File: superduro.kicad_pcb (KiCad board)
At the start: 2 copper layers, 21.6 x 24.1 mm, 16 parts, among them J1 Stomp_Connector, J2 Conn_01x02, J3 Conn_01x01, J4 GND, Q1 BS170

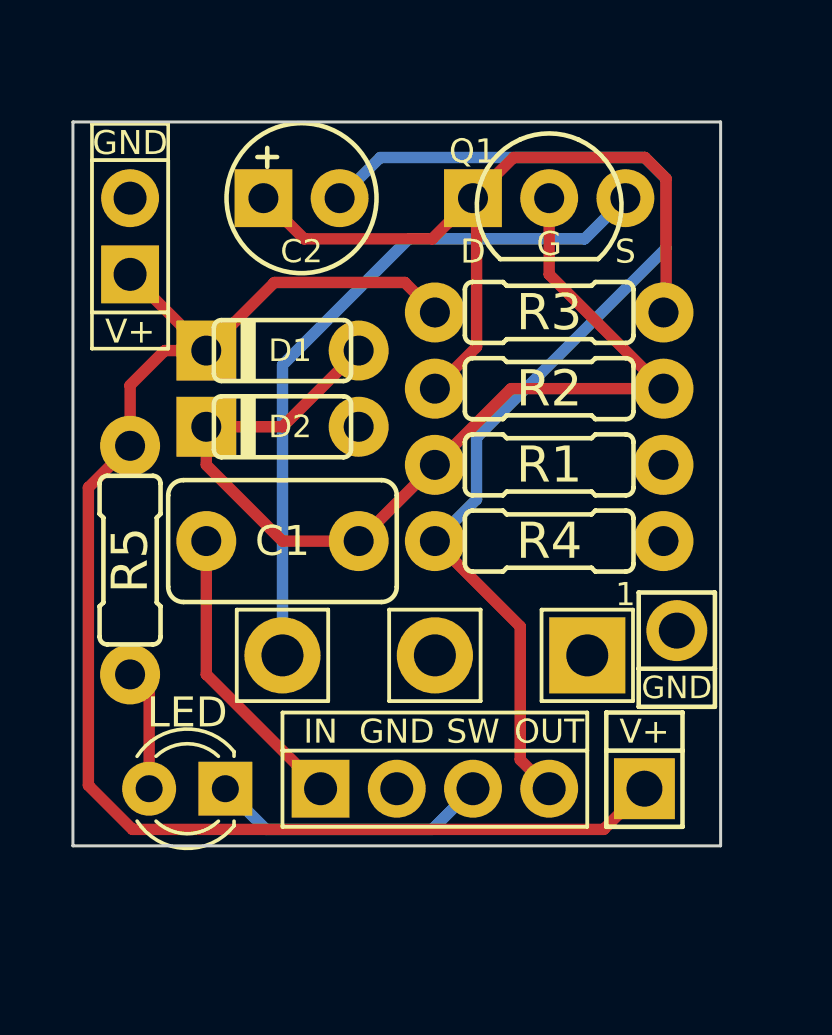
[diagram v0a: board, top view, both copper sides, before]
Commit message: v0.2: Superheated SHO
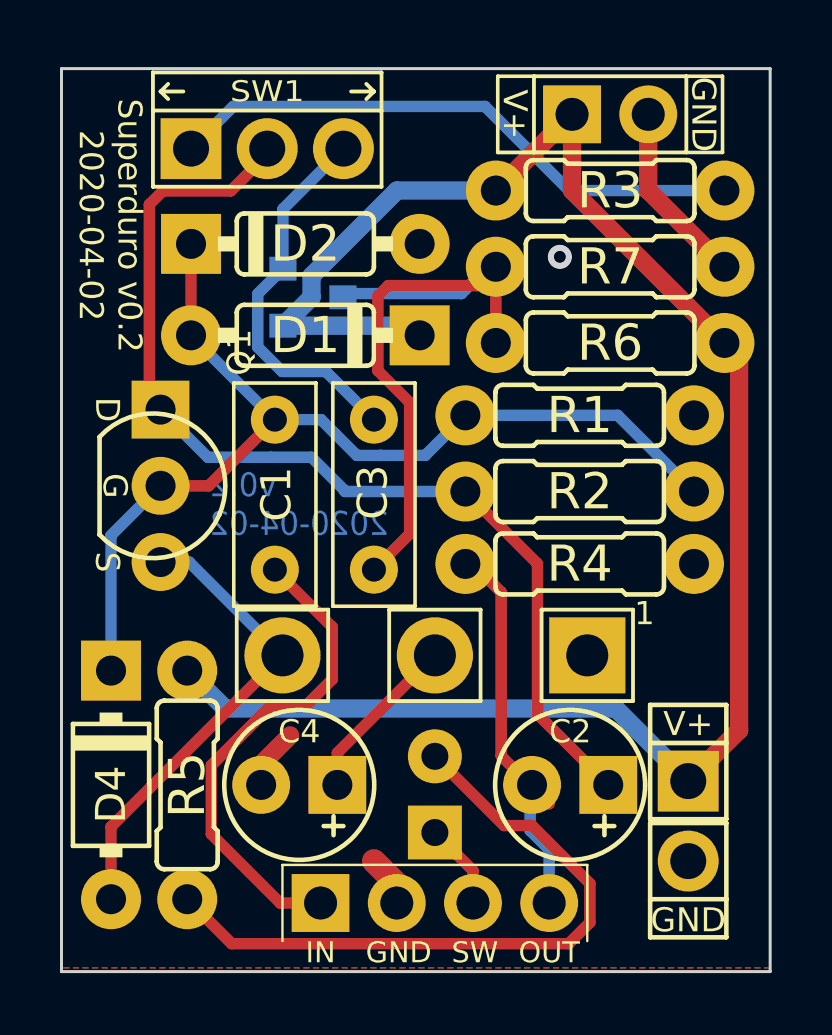
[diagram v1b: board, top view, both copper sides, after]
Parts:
- added C3: 100n, rockola_kicad_footprints:C_Box_7.2_2.5, F.Cu at (71.6, 65.7)
- added C4: 10u, caps-elec:0502, F.Cu at (69.1, 72.9)
- added D4: 9V1, diodes:DO41-3, F.Cu at (62.9, 72.9)
- added Q2: MMBF5457, rockola_kicad_footprints:SOT-23_NJFET_DSG, B.Cu at (69.6, 56.6)
- added R6: 1M, resistors:0.3%22.B, F.Cu at (79.5, 58.2)
- added R7: 1M, resistors:0.3%22.B, F.Cu at (79.5, 55.6)
- added SW1: SW_SPDT, switches:SPDT.WIRE, F.Cu at (68.1, 51.7)
- C1: footprint caps-film:0.2_22.MED -> rockola_kicad_footprints:C_Box_7.2_2.5
- D1, D2: footprint diodes:DO35-2 -> diodes:DO35-3
- D3: moved to B.Cu
- J1: footprint rockola_kicad_footprints:Stomp_4pin -> rockola_kicad_footprints:Stomp_4pin_ALT2
- J4: value GND -> Conn_01x01
- R3: value 5k1 -> 4k7
- RV1: value C5k -> B1k
- moved C2 21.5 mm to (78.2, 72.9), turned to 180 degrees
- moved Q1 16.1 mm to (64.5, 62.9), turned to -90 degrees
- moved J2 15.0 mm to (79.5, 51.8), turned to -90 degrees
- moved R5 7.73 mm to (65.4, 72.9)
- moved J4 7.69 mm to (82.1, 75.4)
- moved D3 7.14 mm to (73.7, 74.5), turned to 90 degrees
- moved D2 6.14 mm to (69.3, 54.9)
- moved R3 4.54 mm to (79.5, 53.1)
- moved J1 3.81 mm to (73.7, 76.8)
- moved R2 3.58 mm to (78.5, 63.1)
- moved R1 1.94 mm to (78.5, 60.6)
- moved J3 1.48 mm to (82.1, 72.8)
- moved R4 1.27 mm to (78.5, 65.5)
- moved C1 0.99 mm to (68.3, 65.7), turned to 90 degrees
- moved D1 0.92 mm to (69.3, 57.9), turned to 180 degrees
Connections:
- R3 pad 2: Net-(C2-Pad1) -> Net-(R3-Pad2)
- RV1 pad 2: GND -> Net-(C4-Pad1)
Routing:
- net OUT: track 36.8 -> 13.3 mm
- net Net-(C3-Pad1): track 0.00 -> 22.4 mm
- net Net-(R3-Pad2): track 0.00 -> 19.5 mm
- net Net-(D3-Pad2): track 4.07 -> 22.5 mm
- net Net-(C3-Pad2): track 0.00 -> 12.7 mm
- net +9V: track 49.2 -> 61.1 mm
- net GND: track 0.00 -> 10.0 mm, vias 0 -> 1
- net Net-(C2-Pad1): track 26.9 -> 34.9 mm
- net Net-(D4-Pad2): track 23.4 -> 16.4 mm
- net IN: track 9.83 -> 16.6 mm
- net LED-: track 9.38 -> 2.88 mm
- net Net-(C4-Pad1): track 0.00 -> 6.20 mm
- net Net-(C1-Pad2): track 33.7 -> 34.7 mm
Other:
- board size 21.6 x 24.1 mm -> 23.6 x 30.1 mm
- board text added: "HOT"
- board text added: "SH"
- board text added: "SW1"
- board text added: "Superduro v0.2 2020-04-02"
- board text added: "v0.2 2020-04-02"
- board text removed: "v0.1 2020-03-21"

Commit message: updated to KiCad 6.0
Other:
- net class Default removed
